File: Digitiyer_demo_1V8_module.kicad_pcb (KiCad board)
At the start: 2 copper layers, 37.8 x 35 mm, 103 parts, among them J1 Conn_01x08, J2 Conn_01x24, J3 Conn_01x04_Pin, J4 USB_C_Receptacle_PowerOnly_6P, Q1 AO3400A, Q2 SI1308EDL, U1 Opamp_Quad, U2 LM27762DSSR, U3 TMUX1108PWR, U4 RF-BM-ND05, U5 TPS63900DSKR, U6 TXB0108PWR, U7 74LVC1G34GW, U8 74LVC1G34GW

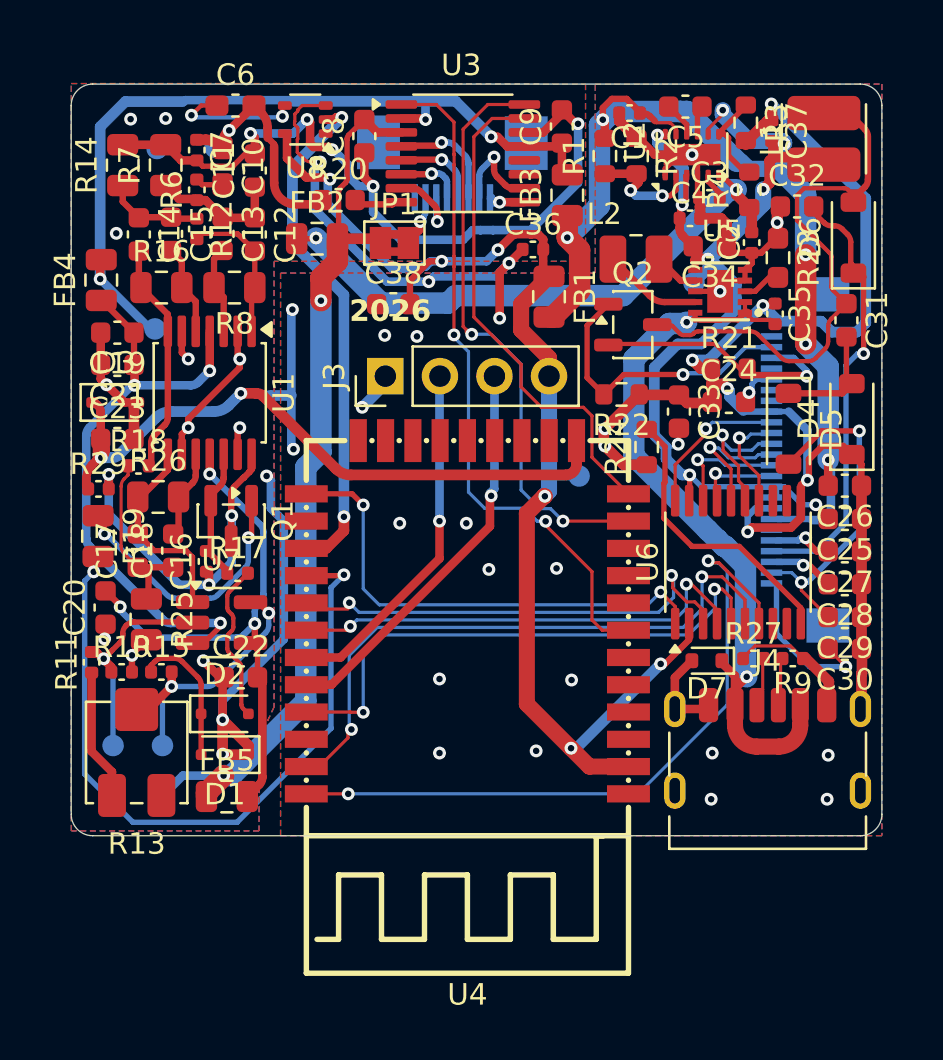
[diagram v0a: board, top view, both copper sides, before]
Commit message: uložitt
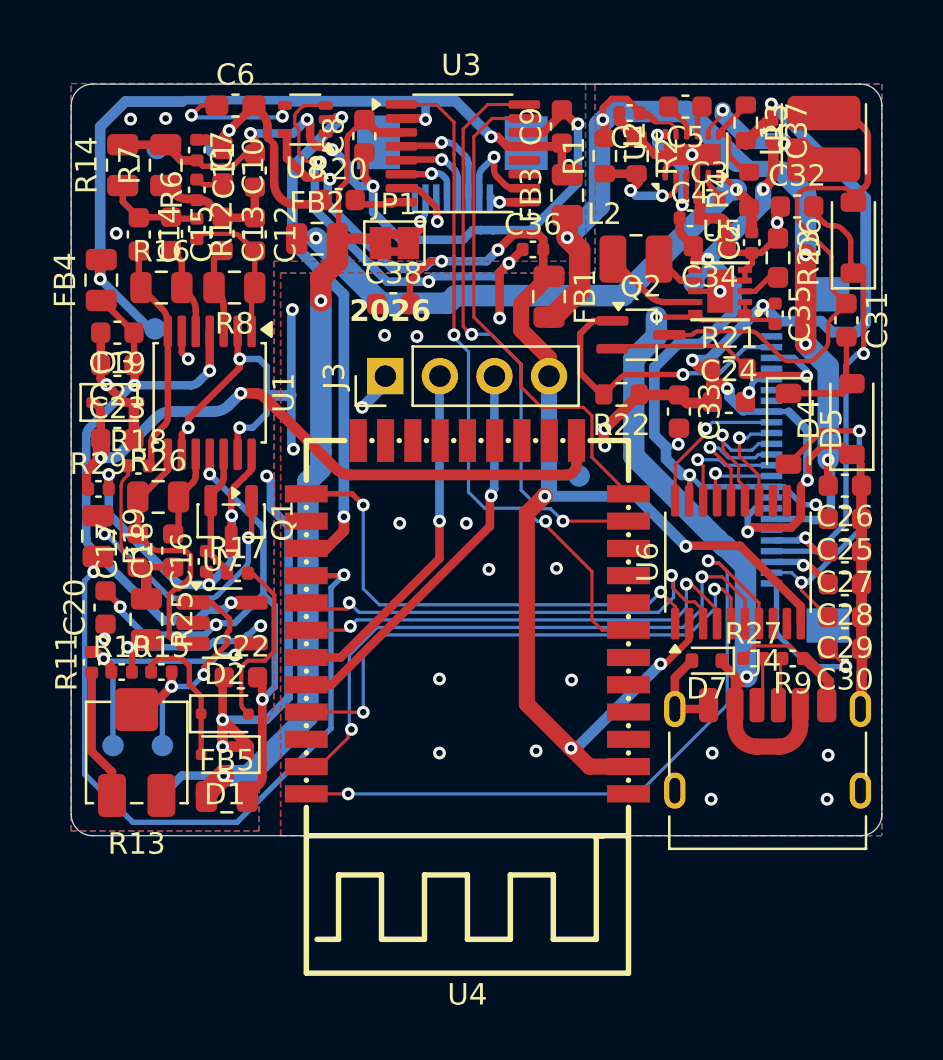
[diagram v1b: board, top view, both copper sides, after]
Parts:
- removed R24: 50k, Resistor_SMD:R_0603_1608Metric
- Q2: footprint Package_TO_SOT_SMD:SOT-23-3 -> Package_TO_SOT_SMD:SOT-323_SC-70_Handsoldering
- U7: value 74LVC1G34GW -> OPA365AQDBVRQ1
- moved Q2 0.61 mm to (178.3, 77.7)
- moved REF** 0.05 mm to (156.0, 99.1)
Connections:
- U6 pad 10: Net-(U6-OE) -> +1V8
- U7 pad 1: /AFE/OP3O -> Net-(R13-Pad2)
- U7 pad 2: Net-(U7--) -> /AFE/OPAMP_-
- U7 pad 3: /AFE/OPAMP_+ -> /AFE/OP3O
- U7 pad 4: /AFE/OPAMP_- -> Net-(U7--)
- U7 pad 5: Net-(R13-Pad2) -> /AFE/OPAMP_+
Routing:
- net +1V8: track 59.1 -> 73.9 mm, vias 6 -> 7
- net Net-(U6-OE): track 13.3 -> 0.00 mm
- net VSSA: track 75.5 -> 87.8 mm
- net /AFE/OP3O: track 9.48 -> 12.7 mm
- net /AFE/OPAMP_-: track 25.9 -> 29.0 mm, vias 3 -> 4
- net GND: track 129.5 -> 127.0 mm
- net Net-(U7--): track 11.3 -> 12.9 mm, vias 1 -> 2
- net Net-(D6-A): track 27.9 -> 26.6 mm
- net +3V3: track 48.8 -> 49.9 mm
- net Net-(D2-A): track 7.49 -> 8.41 mm
- net Net-(D7-C): track 38.3 -> 37.6 mm
- net Net-(R13-Pad2): track 13.0 -> 12.5 mm
- net /AFE/OPAMP_+: track 28.6 -> 28.0 mm
- net VEE: track 42.0 -> 42.5 mm

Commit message: uklad
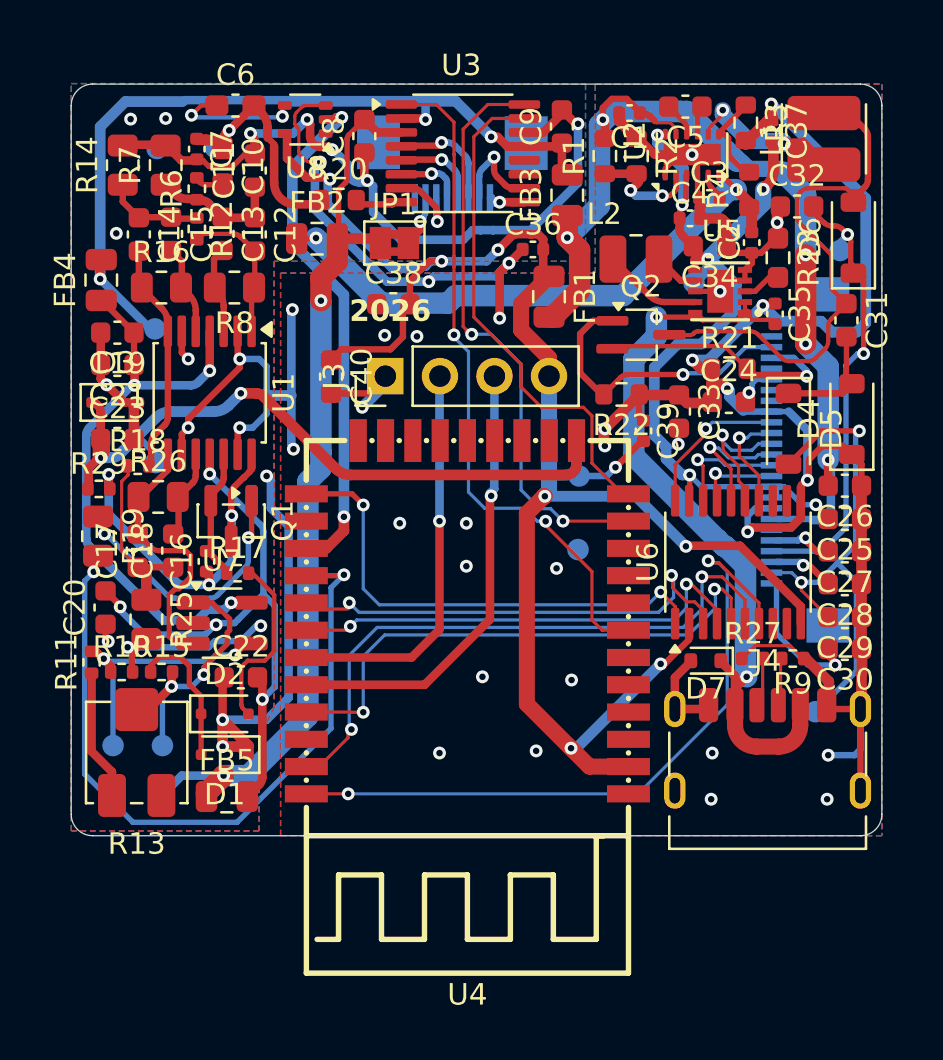
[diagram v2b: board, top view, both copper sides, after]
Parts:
- added C39: 10uF, Capacitor_SMD:C_0402_1005Metric, F.Cu at (178.4, 82.2)
- added C40: 100nF, Capacitor_SMD:C_0603_1608Metric, F.Cu at (163.8, 79.6)
- added REF**: TestPoint_Pad_D1.0mm, TestPoint:TestPoint_Pad_D1.0mm, B.Cu at (187.6, 73.8)
- added REF**: TestPoint_Pad_D1.0mm, TestPoint:TestPoint_Pad_D1.0mm, B.Cu at (175.3, 87.7)
- added REF**: TestPoint_Pad_D1.0mm, TestPoint:TestPoint_Pad_D1.0mm, B.Cu at (155.7, 83.6)
- added REF**: TestPoint_Pad_D1.0mm, TestPoint:TestPoint_Pad_D1.0mm, B.Cu at (186.4, 95.2)
- R10, R11, R12, R15, R17, R18, R27, R29, R6, R9: footprint Capacitor_SMD:C_0402_1005Metric -> Resistor_SMD:R_0402_1005Metric
- R14, R16, R19, R25, R26, R7, R8: footprint Capacitor_SMD:C_0805_2012Metric -> Resistor_SMD:R_0805_2012Metric
- R20: footprint Capacitor_SMD:C_0603_1608Metric -> Resistor_SMD:R_0603_1608Metric
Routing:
- net GND: track 127.0 -> 140.2 mm
- net +1V8: track 73.9 -> 83.0 mm, vias 7 -> 8
- net /PREVGL: track 15.8 -> 24.1 mm
- net /SWCLK: track 18.7 -> 21.3 mm
- net /SWDIO: track 16.6 -> 18.5 mm
- net INTG: track 31.3 -> 32.9 mm
- net /PREVGH: track 20.5 -> 21.5 mm, vias 1 -> 2
- net /VCOM: track 7.35 -> 6.51 mm
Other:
- board text added: "INTG"

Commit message: finální uložení?
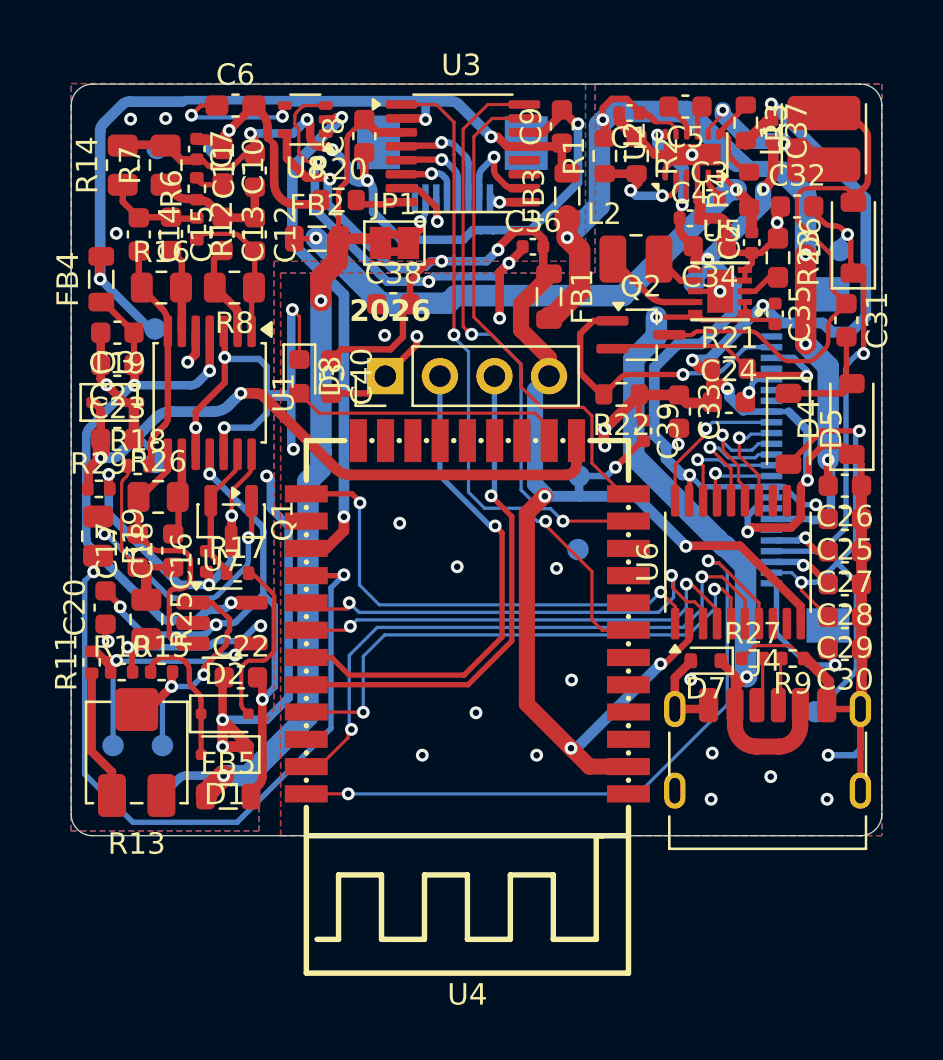
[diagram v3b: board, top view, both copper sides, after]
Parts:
- added D8: LED_Small, LED_SMD:LED_0603_1608Metric, F.Cu at (162.4, 79.6)
- FB1, FB2, FB3, FB4, FB5: footprint Capacitor_SMD:C_0805_2012Metric -> Inductor_SMD:L_0805_2012Metric
- U1: value Opamp_Quad -> COS8054TR
- moved C36 0.13 mm to (173.3, 73.6)
- moved FB5 0.06 mm to (159.1, 99.2)
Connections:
- U1 pad 10: /AFE/OP3M -> VSSA
- U1 pad 12: /AFE/OP4M -> VSSA
- U1 pad 13: VSSA -> /AFE/OP4M
- U1 pad 2: VSSA -> /AFE/OP1M
- U1 pad 3: /AFE/OP1M -> VSSA
- U1 pad 5: /AFE/OP2M -> VSSA
- U1 pad 6: VSSA -> /AFE/OP2M
- U1 pad 9: VSSA -> /AFE/OP3M
- U4 pad 14: unconnected-(U4-P03-Pad14) -> Net-(D8-A)
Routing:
- net Net-(D8-A): track 0.00 -> 12.9 mm
- net /SWDIO: track 18.5 -> 23.7 mm
- net GND: track 140.2 -> 143.5 mm
- net /SWCLK: track 21.3 -> 23.3 mm
- net VSSA: track 87.6 -> 88.2 mm
- net /AFE/OP4M: track 6.27 -> 6.80 mm
- net /AFE/OP1M: track 4.07 -> 4.58 mm
